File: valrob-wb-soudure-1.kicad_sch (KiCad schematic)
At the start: 29 parts, among them J1 Conn_01x03, J2 Conn_01x06, J6 Conn_01x02, J7 Conn_01x02, Q1 2N7000, SW2 SW_Push, SW3 SW_Push, SW4 SW_Push, SW5 SW_Push

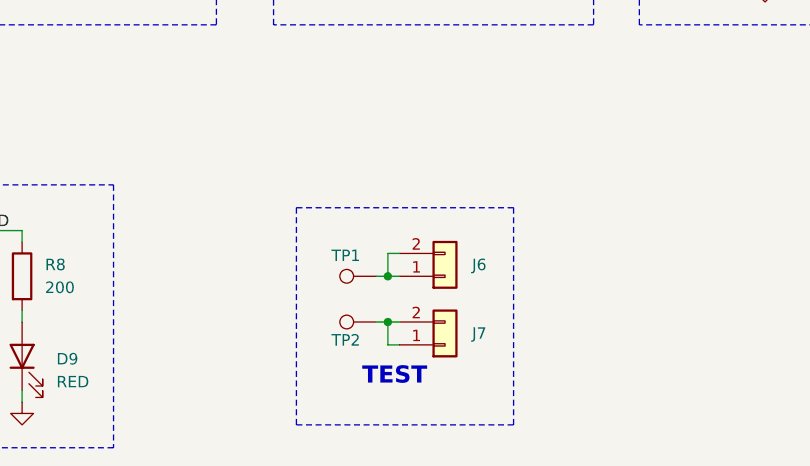
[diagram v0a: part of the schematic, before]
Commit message: schem: add jst connectors to test
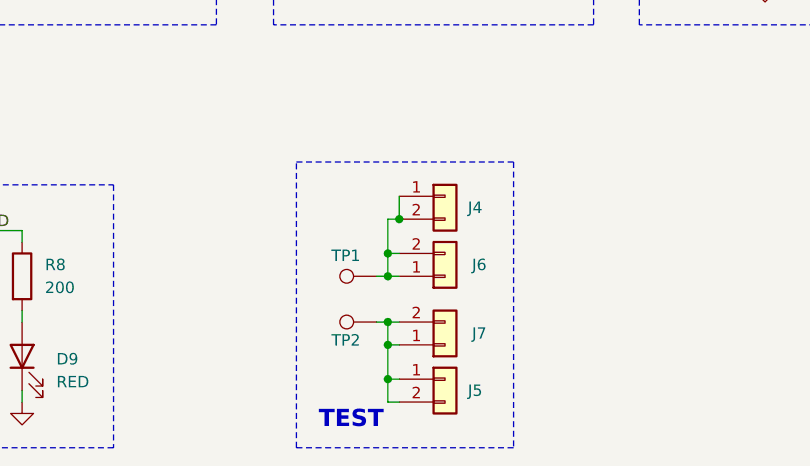
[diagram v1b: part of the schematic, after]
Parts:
- added J4, J5: Conn_01x02, Connector_JST:JST_XH_B2B-XH-A_1x02_P2.50mm_Vertical, symbol Connector_Generic:Conn_01x02
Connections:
- net at J6.1 (Pin_1), J6.2 (Pin_2), TP1.1: now also J4.1 (Pin_1), J4.2 (Pin_2)
- net at J7.1 (Pin_1), J7.2 (Pin_2), TP2.1: now also J5.1 (Pin_1), J5.2 (Pin_2)
